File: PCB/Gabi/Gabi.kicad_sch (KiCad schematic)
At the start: 16 parts

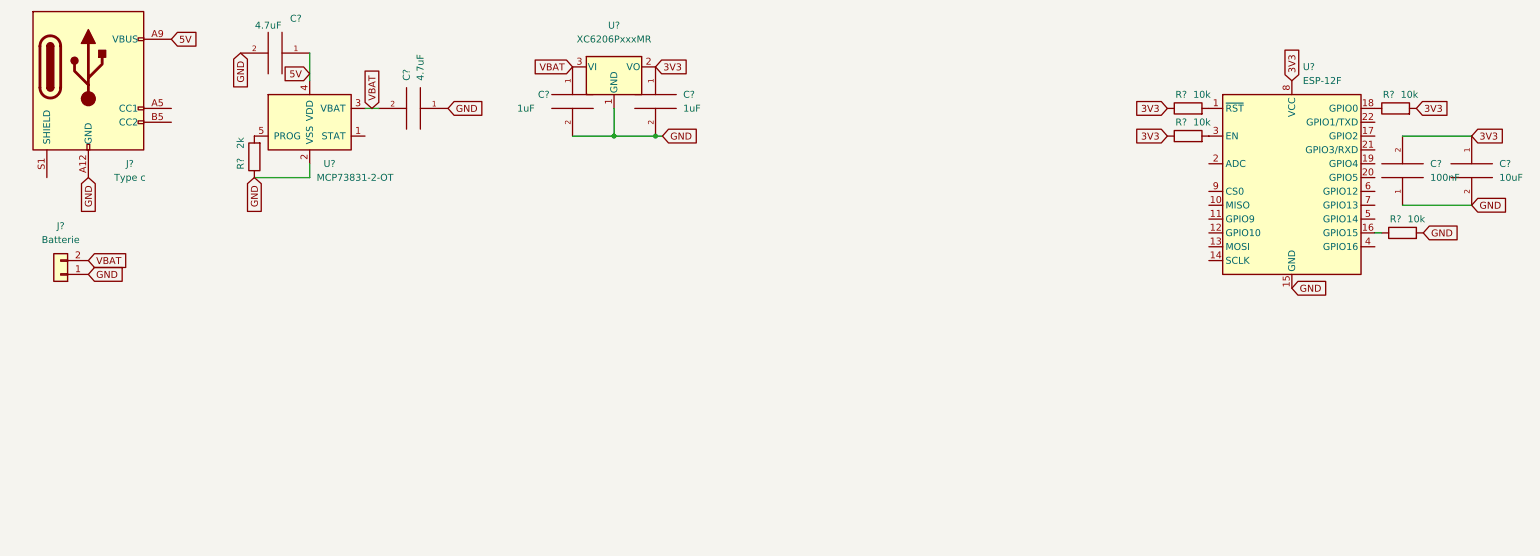
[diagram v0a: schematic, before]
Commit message: PCB UPDATE
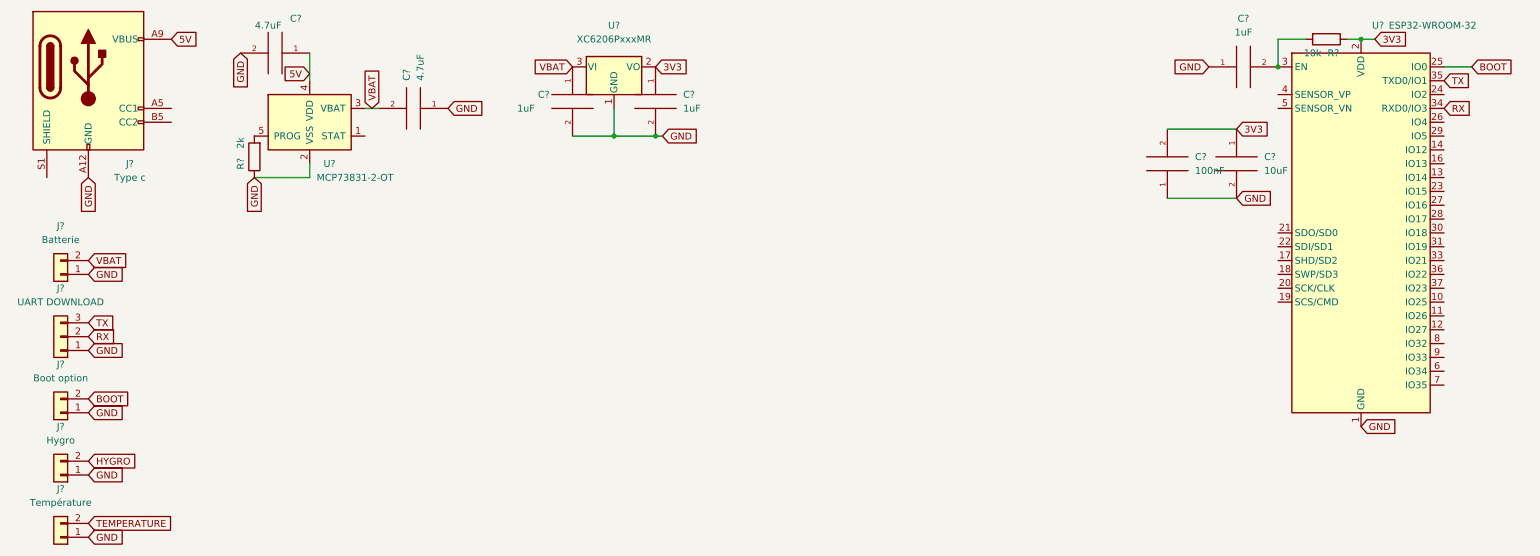
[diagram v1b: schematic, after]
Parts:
- removed C?: 10uF, symbol pspice:C
- removed C?: 100nF, symbol pspice:C
- removed R? (x4): 10k, symbol Device:R
- removed U?: ESP-12F, RF_Module:ESP-12E, symbol RF_Module:ESP-12F
- added C?: 1uF, Capacitor_SMD:C_0805_2012Metric, symbol pspice:C
- added C?: 10uF, Capacitor_SMD:C_0805_2012Metric, symbol pspice:C
- added C?: 100nF, Capacitor_SMD:C_0805_2012Metric, symbol pspice:C
- added J?: Hygro, Connector_PinHeader_2.54mm:PinHeader_1x02_P2.54mm_Vertical, symbol Connector_Generic:Conn_01x02
- added J?: UART DOWNLOAD, Connector_PinHeader_2.54mm:PinHeader_1x03_P2.54mm_Vertical, symbol Connector_Generic:Conn_01x03
- added J?: Température, Connector_PinHeader_2.54mm:PinHeader_1x02_P2.54mm_Vertical, symbol Connector_Generic:Conn_01x02
- added J?: Boot option, Connector_PinHeader_2.54mm:PinHeader_1x02_P2.54mm_Vertical, symbol Connector_Generic:Conn_01x02
- added R?: 10k, Resistor_SMD:R_0805_2012Metric, symbol Device:R
- added U?: ESP32-WROOM-32, RF_Module:ESP32-WROOM-32, symbol RF_Module:ESP32-WROOM-32
- C? (x4): footprint (none) -> Capacitor_SMD:C_0805_2012Metric
- J?: footprint (none) -> Connector_PinHeader_2.54mm:PinHeader_1x02_P2.54mm_Vertical
- R?: footprint (none) -> Resistor_SMD:R_0805_2012Metric
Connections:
- net 3V3: now also C?.1, C?.2, R?.1, U?.2 (VDD)
- net GND: now also C?.1, C?.1, C?.2, J?.1 (Pin_1), J?.1 (Pin_1), J?.1 (Pin_1), J?.1 (Pin_1), U?.1 (GND), U?.15 (GND), U?.38 (GND), U?.39 (GND)
- new net: C?.2, R?.2, U?.3 (EN)
- new net BOOT: J?.2 (Pin_2), U?.25 (IO0)
- new net HYGRO: J?.2 (Pin_2)
- new net RX: J?.2 (Pin_2), U?.34 (RXD0/IO3)
- new net TEMPERATURE: J?.2 (Pin_2)
- new net TX: J?.3 (Pin_3), U?.35 (TXD0/IO1)
